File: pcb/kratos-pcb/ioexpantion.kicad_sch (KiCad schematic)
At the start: 2 parts, among them IC2 SN74HC595N, IC3 ULN2003A

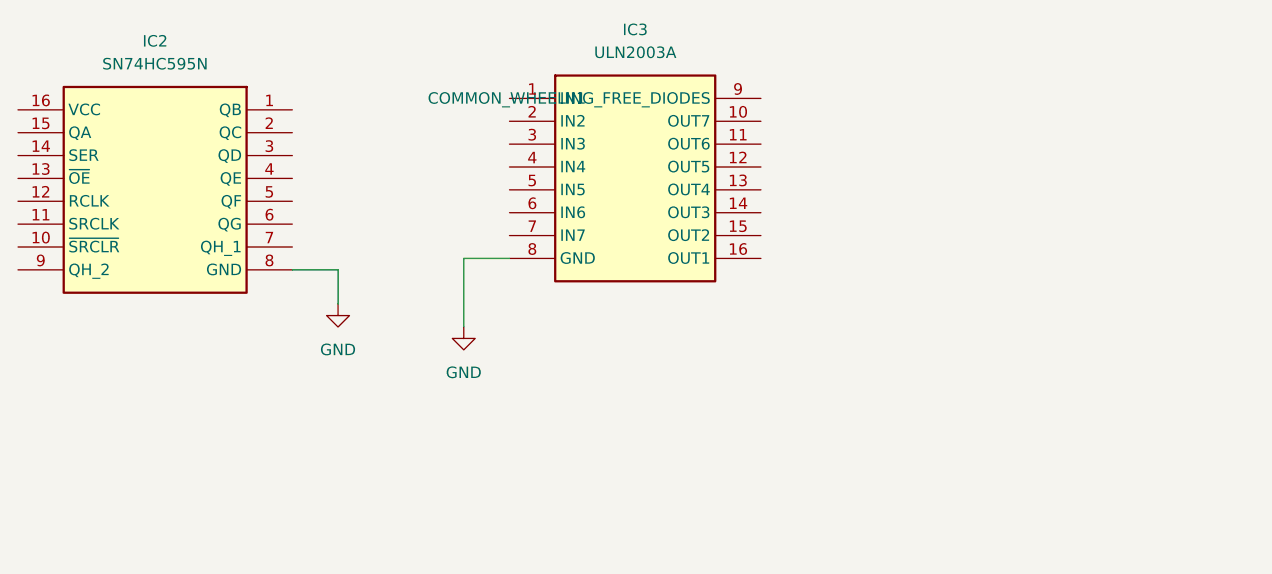
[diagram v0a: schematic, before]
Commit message: ### added
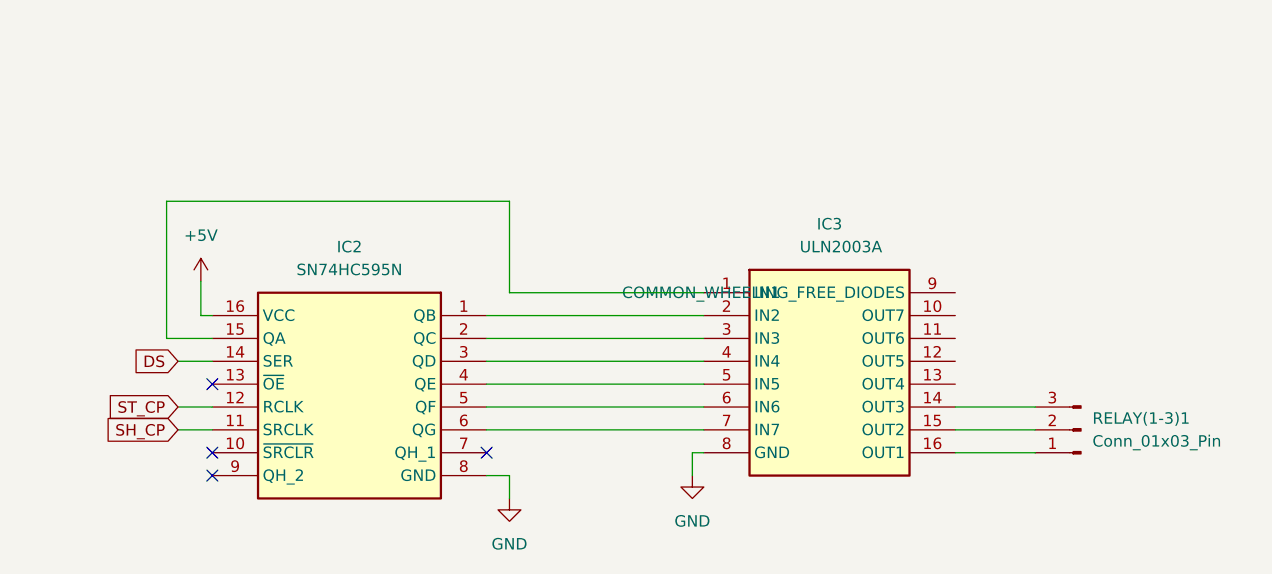
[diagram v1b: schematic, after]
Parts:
- added RELAY(1-3)1: Conn_01x03_Pin, symbol Connector:Conn_01x03_Pin
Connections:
- net at IC3.1 (IN1): now also IC2.15 (QA)
- net at IC3.14 (OUT3): now also RELAY(1-3)1.3 (Pin_3)
- net at IC3.15 (OUT2): now also RELAY(1-3)1.2 (Pin_2)
- net at IC3.16 (OUT1): now also RELAY(1-3)1.1 (Pin_1)
- net at IC3.2 (IN2): now also IC2.1 (QB)
- net at IC3.3 (IN3): now also IC2.2 (QC)
- net at IC3.4 (IN4): now also IC2.3 (QD)
- net at IC3.5 (IN5): now also IC2.4 (QE)
- net at IC3.6 (IN6): now also IC2.5 (QF)
- net at IC3.7 (IN7): now also IC2.6 (QG)
- net SH_CP: now reaches IC2.11 (SRCLK)
- net ST_CP: now reaches IC2.12 (RCLK)
- net DS: now reaches IC2.14 (SER)
- net +5V: now reaches IC2.16 (VCC)
- no-connect marks 0 -> 4
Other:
- moved on the sheet: IC2, IC3
